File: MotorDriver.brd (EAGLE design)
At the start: 115.4 x 156.7 mm, 145 parts, among them IC3 STM32F071V8T6V8, J10 B4B-PH-K-S(LF)(SN), J11 B4B-PH-K-S(LF)(SN), J12 B4B-PH-K-S(LF)(SN), J13 B4B-PH-K-S(LF)(SN), J14 B4B-PH-K-S(LF)(SN), J15 B4B-PH-K-S(LF)(SN), J16 B4B-PH-K-S(LF)(SN), J18 B2P-VH(LF)(SN), J19 B2P-VH(LF)(SN), J20 B2P-VH(LF)(SN), J21 B2P-VH(LF)(SN), J22 B2P-VH(LF)(SN), J23 B2P-VH(LF)(SN), J24 B2P-VH(LF)(SN), J25 B2P-VH(LF)(SN), J26 XT30PWXT30PW, J9 B4B-PH-K-S(LF)(SN), M0 VNH7100ASTR, M1 VNH7100ASTR, M2 VNH7100ASTR, M3 VNH7100ASTR, M4 VNH7100ASTR, M5 VNH7100ASTR, M6 VNH7100ASTR, M7 VNH7100ASTR, Q2 20V/4.2A/52mΩ/1.4W, U1 ICE5LP1K-SG48ITR, U10 LD1085D2T33R, U11 LD1085D2T33R, U2 N25Q032A13ESC40F, U3 BD9D323QWZ-E2, U4 BD9D323QWZ-E2, U5 MMDT5401-7-F, U6 BD9D323QWZ-E2, U7 MIC5504-3.3YM5-TR, U8 MIC5365-1.2YC5-TR, U9 LD1085D2T33R, X1 MINI-USB-UX60-MB-5S8, Y1 ECS-TXO-2520-33-160-AN-TR, Y2 32.768kHz, Y4 CRYSTAL-GROUNDEDSMD-3.2X2.5

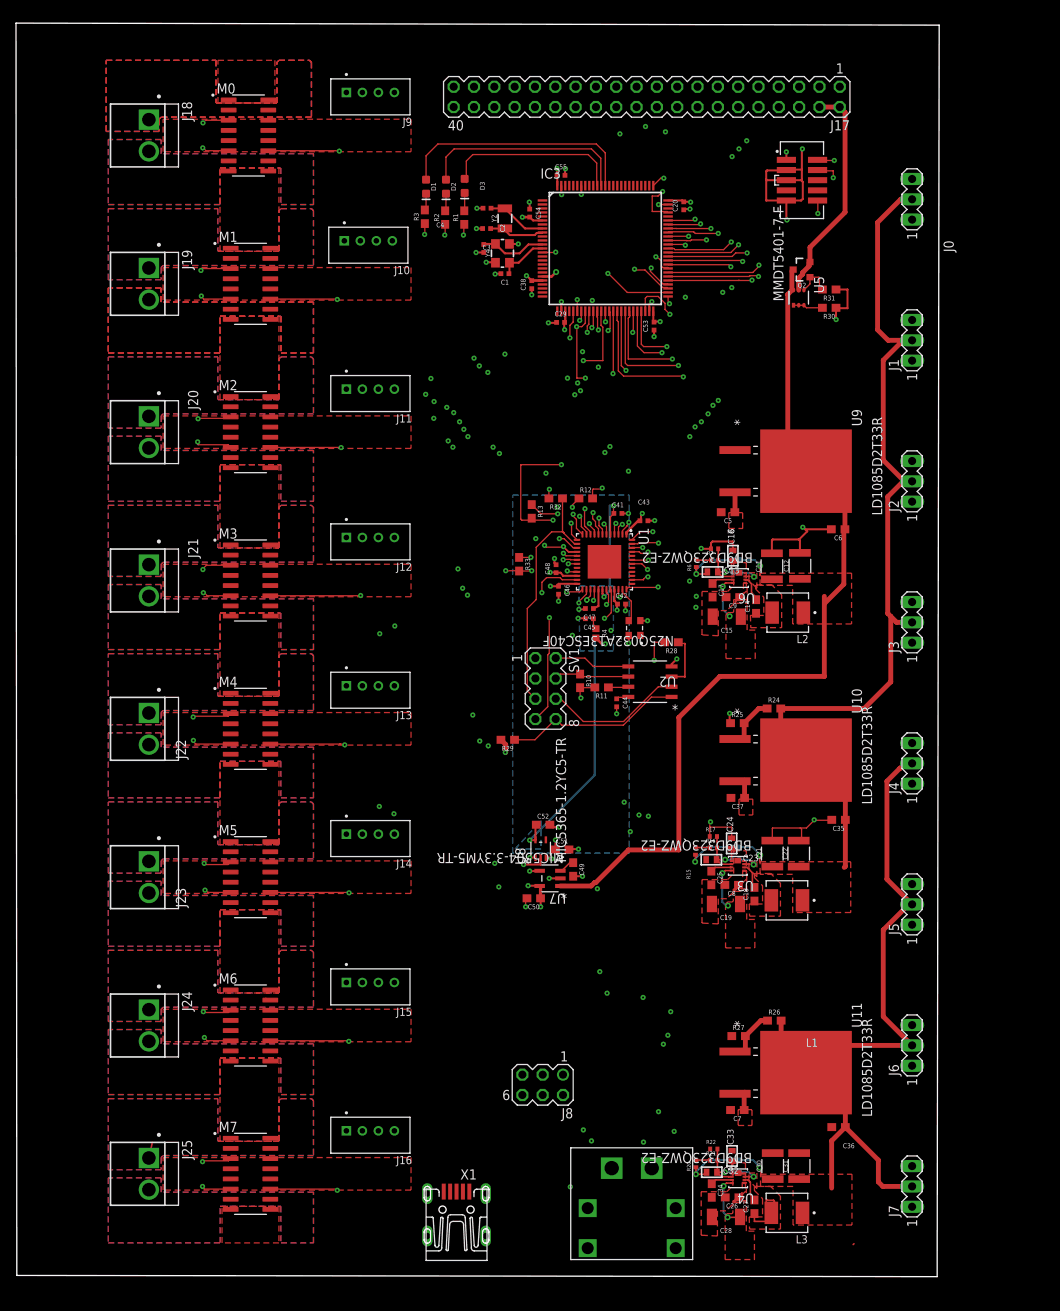
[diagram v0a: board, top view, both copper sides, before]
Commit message: Adding Eagle Files
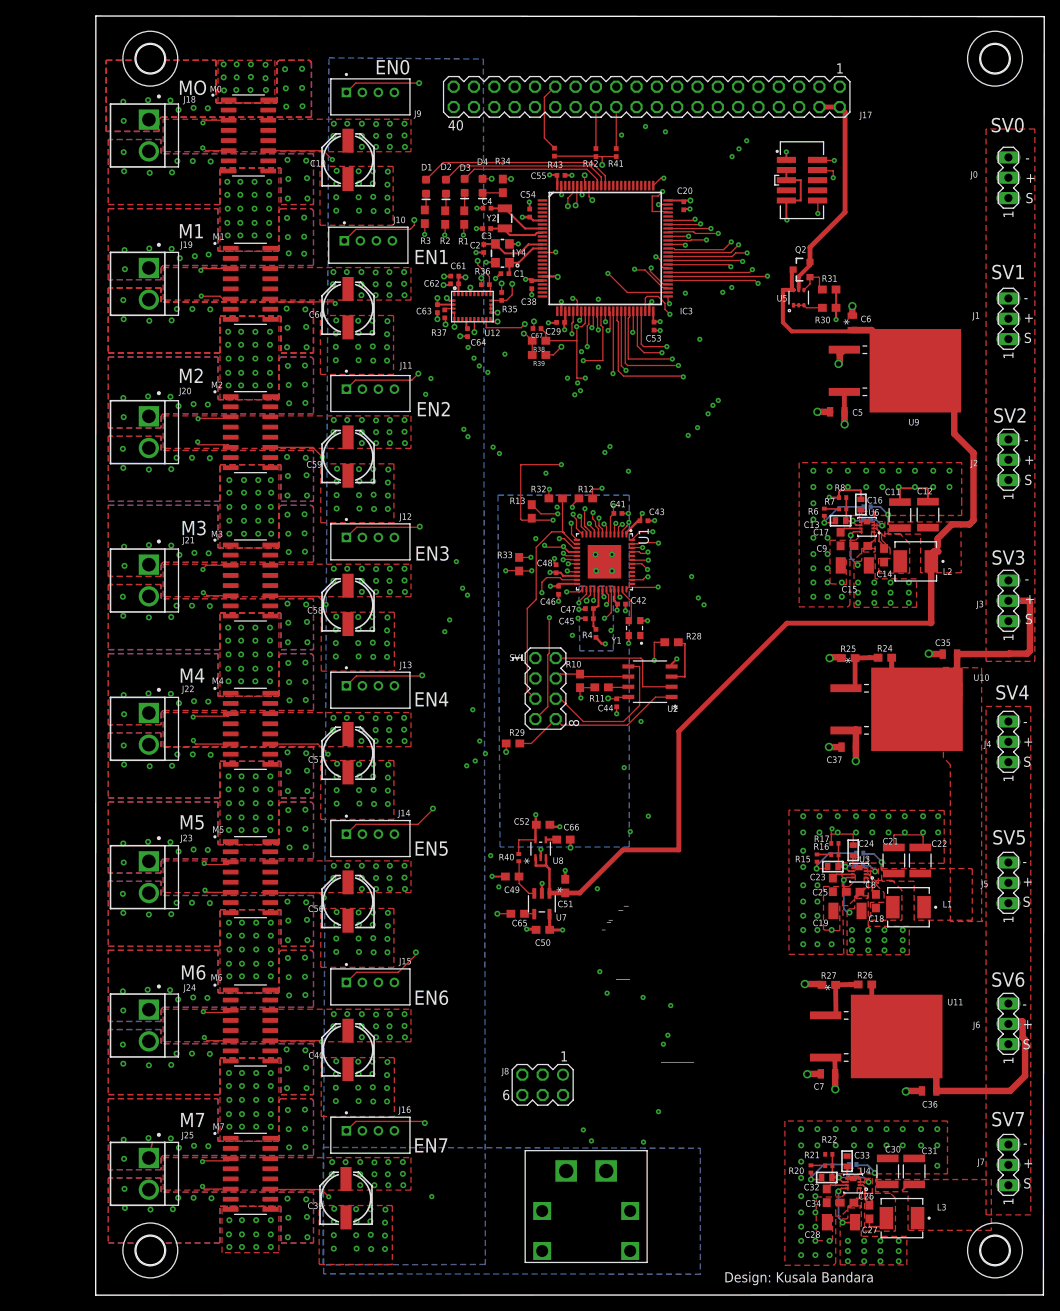
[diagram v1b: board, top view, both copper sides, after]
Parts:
- removed X1: MINI-USB-UX60-MB-5S8, con-hirose:UX60-MB-5S8
- added C10, C39, C40, C56, C57, C58, C59, C60: 100uF, SparkFun-Capacitors:PANASONIC_D
- added C61: 120nF, SparkFun-Capacitors:0402-TIGHT
- added C62: 6.8nF, SparkFun-Capacitors:0402-TIGHT
- added C63, C64: 100nF, SparkFun-Capacitors:0402-TIGHT
- added C65, C66: 1.0uF, SparkFun-Capacitors:0603
- added C67: 1.0uF, SparkFun-Capacitors:0402-TIGHT
- added D4: (no value), SparkFun-LED:LED-0603
- added H1, H2, H3, H4: MOUNT-HOLE3.6, holes:3,6
- added R34: 330, SparkFun-Resistors:0603
- added R35, R36, R41, R42, R43: 47k, SparkFun-Resistors:0402-TIGHT
- added R37: 10k, SparkFun-Resistors:0402-TIGHT
- added R38, R39: 10k, SparkFun-Resistors:0603
- added R40: MCR01MZPF1801, MCR01MZPF1801:RESC1005X40N
- added U12: BNO055, BNO055:LGA28R50P4X10_380X520X100
- C35, C36, C37, C5, C6, C7: device SparkFun-Capacitors:0603 -> SparkFun-Capacitors:0805
- R4: device SparkFun-Resistors:0402 -> SparkFun-Resistors:0402-TIGHT
- moved C6 25.9 mm to (104.2, 99.5), turned to 90 degrees
- moved C35 25.0 mm to (116.4, 58.1)
- moved C5 18.6 mm to (102.3, 88.4)
- moved U9 18.6 mm to (112.1, 93.5)
- moved R5 17.5 mm to (106.0, 76.5)
- moved R9 17.5 mm to (106.0, 74.9)
- moved C13 17.2 mm to (102.7, 74.8)
- moved C17 17.2 mm to (102.7, 72.5)
- moved C11 17.2 mm to (110.1, 75.5)
- moved C16 17.2 mm to (105.3, 76.8)
- moved C9 17.2 mm to (105.3, 71.6)
- moved R7 17.2 mm to (103.0, 76.3)
- moved U6 17.2 mm to (106.0, 74.0)
- moved C12 17.2 mm to (113.6, 75.5)
- moved C14 17.2 mm to (108.2, 70.5)
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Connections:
- removed net 3.3V: C20.2, IC3.75
- new net GYRO_RESET: IC3.93, U12.11
- new net I2C1_SCL: IC3.95, R35.1, U12.19
- new net I2C1_SDA: IC3.96, R36.1, U12.20
- new net INT: IC3.92, U12.14
- new net N$10: C66.1, U8.4
- new net N$11: C65.1, U7.4
- new net N$12: J17.24, R41.1
- new net N$19: J17.26, R42.1
- new net N$38: J17.29, R43.2
- new net N$5: D4.C, R34.2
- new net N$6: R37.2, U12.4
- new net N$9: C64.2, U12.9
- new net PIN10: U12.10
- net FLASH_MISO: now also J8.4, U2.5; no longer J8.3, U2.2
- net FLASH_MOSI: now also J8.3, U2.2; no longer J8.4, U2.5
- net FPGA_CDONE: now also R39.1
- net FPGA_CRESET_B: now also C67.1, R38.1
- net GND: now also C10.-, C39.-, C40.-, C56.-, C57.-, C58.-, C59.-, C60.-, C61.1, C62.1, C63.1, C64.1, C65.2, C66.2, C67.2, R34.1, U12.15, U12.16, U12.17, U12.18, U12.2, U12.25, U12.5, U12.6
- net N$7: now also R40.1
- net RPI_CS: now also R41.2, R42.2, R43.1; no longer J17.29
- net RPI_STATUS: now also IC3.57; no longer IC3.55
- net RPI_USART_RX: now also IC3.55; no longer IC3.57
- net VCC_12V: now also C10.+, C39.+, C40.+, C56.+, C57.+, C58.+, C59.+, C60.+
- net VCC_1_2V: now also R40.2
- net VCC_3.3V: now also C20.2, C61.2, C62.2, C63.2, D4.A, IC3.75, R35.2, R36.2, R37.1, R38.2, R39.2, U12.28, U12.3; no longer C51.1, U7.4, U8.1, U8.3
- net VCC_5V: now also C51.1, U8.1, U8.3
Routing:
- net GND: track 111.9 -> 195.7 mm, vias 45 -> 464
- net VCC_5V: track 111.1 -> 168.3 mm
- net SERVO_A_6V: track 106.6 -> 51.3 mm
- net SERVO_B_6V: track 100.1 -> 45.9 mm
- net GYRO_RESET: track 0.00 -> 36.3 mm, vias 0 -> 2
- net VCC_1_2V: track 49.8 -> 13.9 mm
- net INT: track 0.00 -> 31.8 mm, vias 0 -> 2
- net EN5-B: track 38.0 -> 67.4 mm
- net I2C1_SDA: track 0.00 -> 25.5 mm, vias 0 -> 2
- net I2C1_SCL: track 0.00 -> 23.9 mm, vias 0 -> 2
- net EN4-B: track 86.9 -> 64.8 mm
- net SV2_PWM2: track 50.0 -> 70.4 mm
- net EN4-A: track 83.9 -> 68.4 mm
- net VCC_3.3V: track 47.0 -> 59.2 mm, vias 20 -> 24
- net SV1_PWM1: track 47.5 -> 59.3 mm
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- added copper zone on layer 2, net NP0
- added copper zone on layer 16, net VCC_12V
- added copper zone on layer 3, net VCC_12V
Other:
- board size 115.4 x 156.7 mm -> 118.6 x 159.9 mm
- board text added: "+"
- board text added: "-"
- board text added: "Design: Kusala Bandara"
- board text added: "EN0"
- board text added: "EN1"
- board text added: "EN2"
- board text added: "EN3"
- board text added: "EN4"
- board text added: "EN5"
- board text added: "EN6"
- board text added: "EN7"
- board text added: "M1"
- board text added: "M2"
- board text added: "M3"
- board text added: "M4"
- board text added: "M5"
- board text added: "M6"
- board text added: "M7"
- board text added: "MO"
- board text added: "S"
- board text added: "SV0"
- board text added: "SV1"
- board text added: "SV2"
- board text added: "SV3"
- board text added: "SV4"
- board text added: "SV5"
- board text added: "SV6"
- board text added: "SV7"
